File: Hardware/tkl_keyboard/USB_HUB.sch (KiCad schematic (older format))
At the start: 20 parts, among them U4 TUSB2046b, U6 SRV05-4, U8 SRV05-4, X1 625L3C006M00000

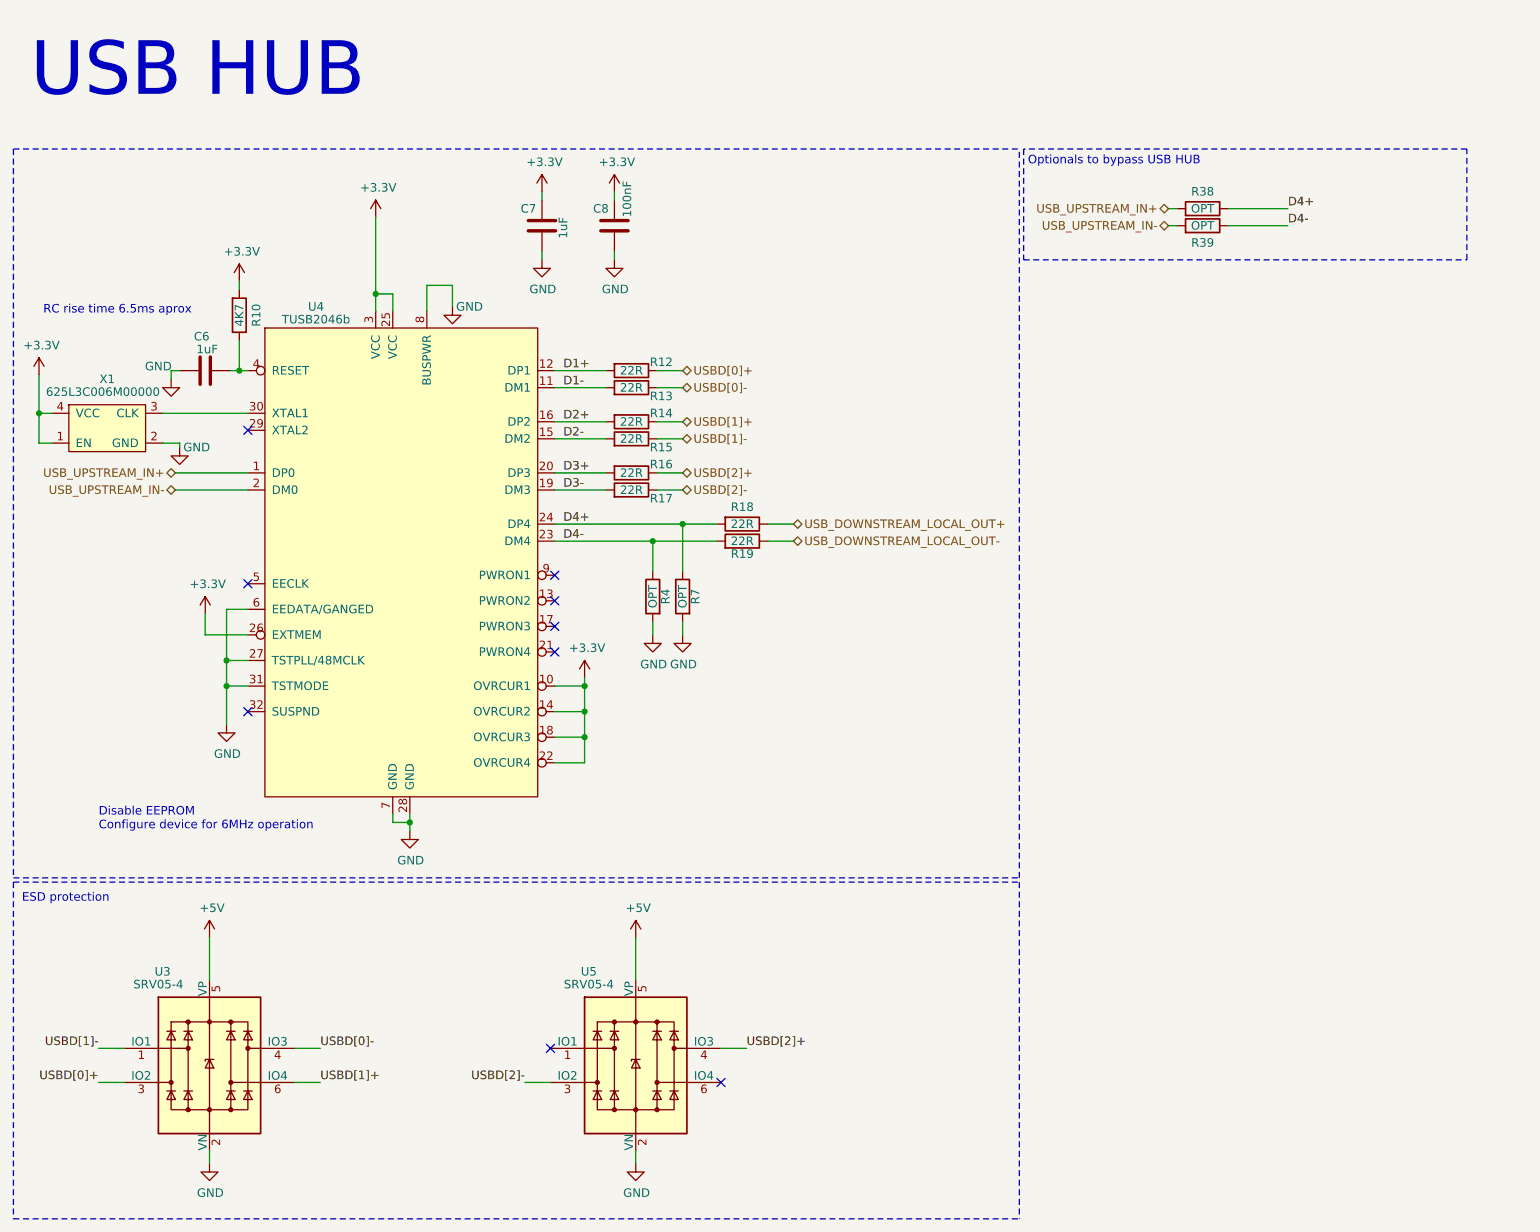
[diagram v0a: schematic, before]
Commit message: Generating gerbers
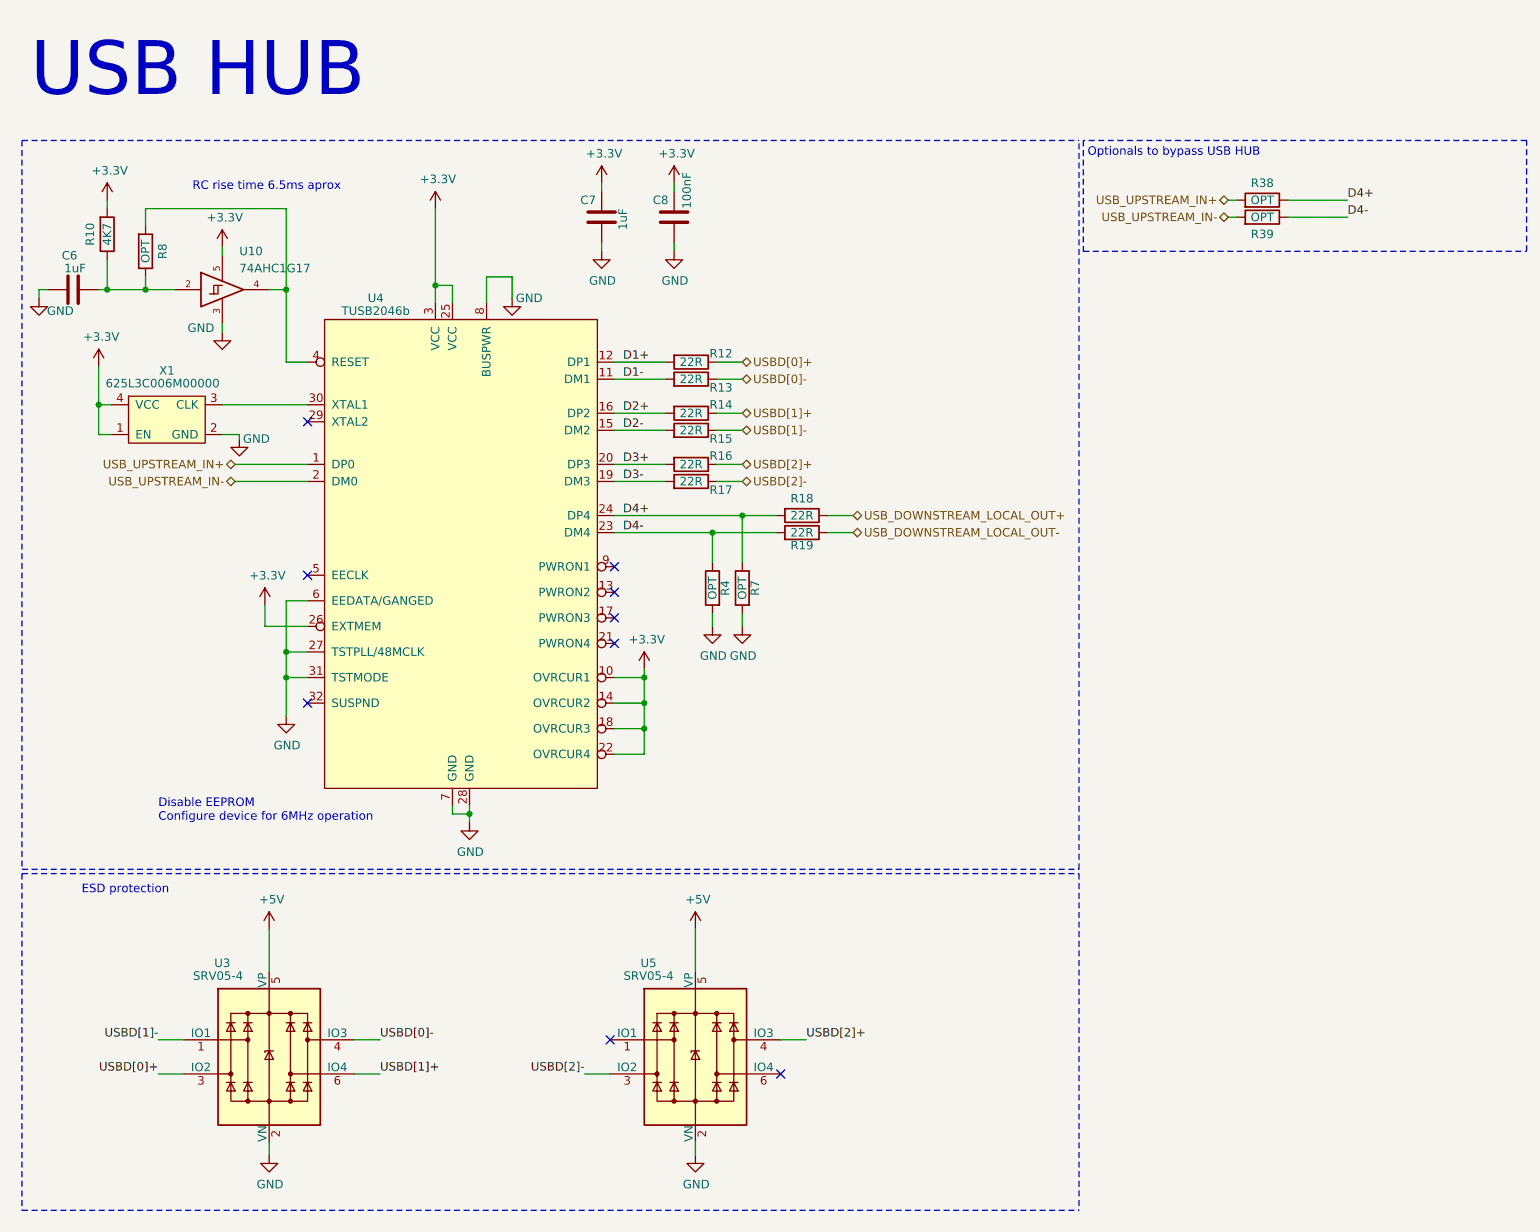
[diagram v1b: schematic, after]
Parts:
- added R8: OPT, resistor_smd:R_0603_1608Metric, symbol Device:R
- added U10: 74AHC1G17, Package_TO_SOT_SMD:SOT-353_SC-70-5, symbol custom_parts_library:74AHC1G17
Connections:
- net +3V3: now also U10.5
- net GND: now also U10.3
- net at C44.2, R1.1: now also R8.1, U10.2; no longer U4.4 (RESET)
- new net: R8.2, U10.4, U4.4 (RESET)
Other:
- moved on the sheet: C6, C7, C8, R10, R12, R13, R14, R15, R16, R17, R18, R19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
